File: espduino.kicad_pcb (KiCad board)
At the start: 2 copper layers, 62 x 65 mm, 29 parts, among them CON101 USB-MICRO-B, IC101 ATMEGA168-A, P101 CONN_01X12, P102 CONN_01X12, P103 FTDI, P104 CONN_01X02, P401 CONN_01X02, P402 CONN_01X02, SW101 SPST, U201 74HCT125, U202 7400, U301 LSF0204x, U302 ESP8266, U401 LD1117S12TR, U402 LD1117S33TR, X101 16Mhz

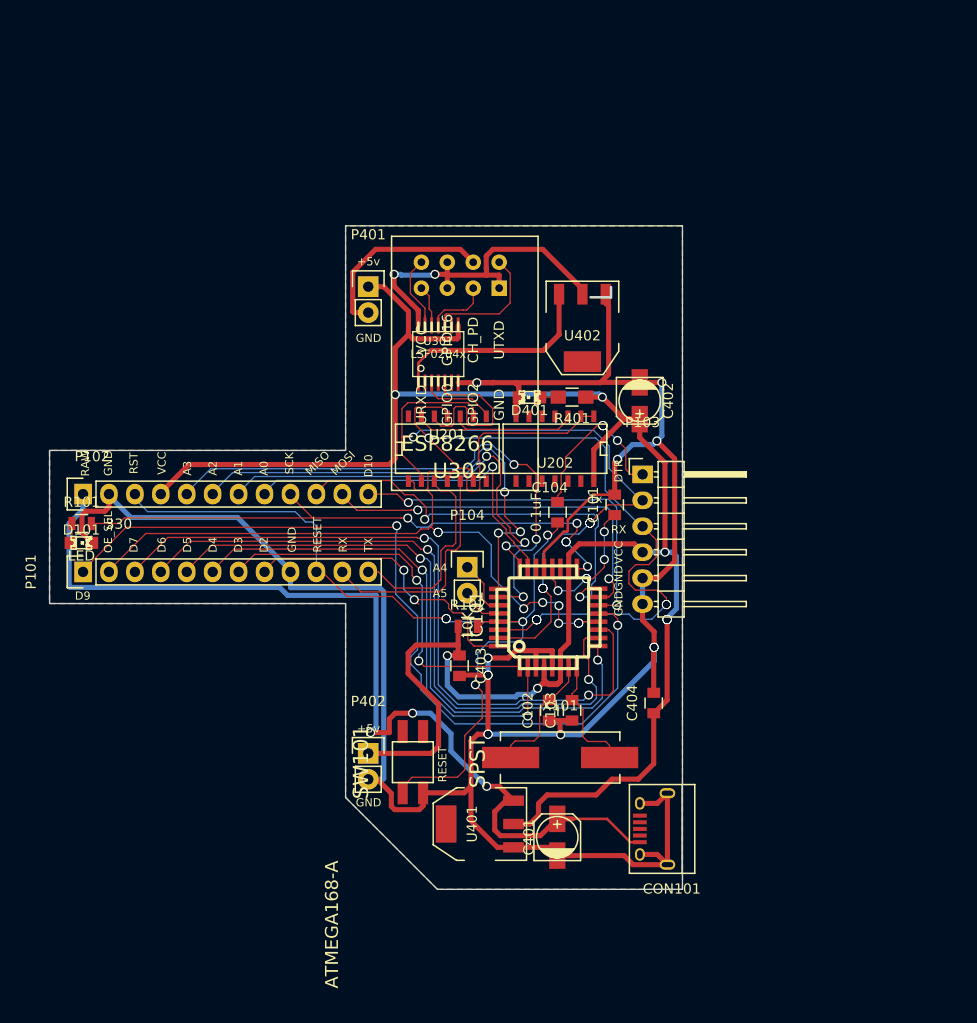
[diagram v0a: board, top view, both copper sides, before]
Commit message: More fixes
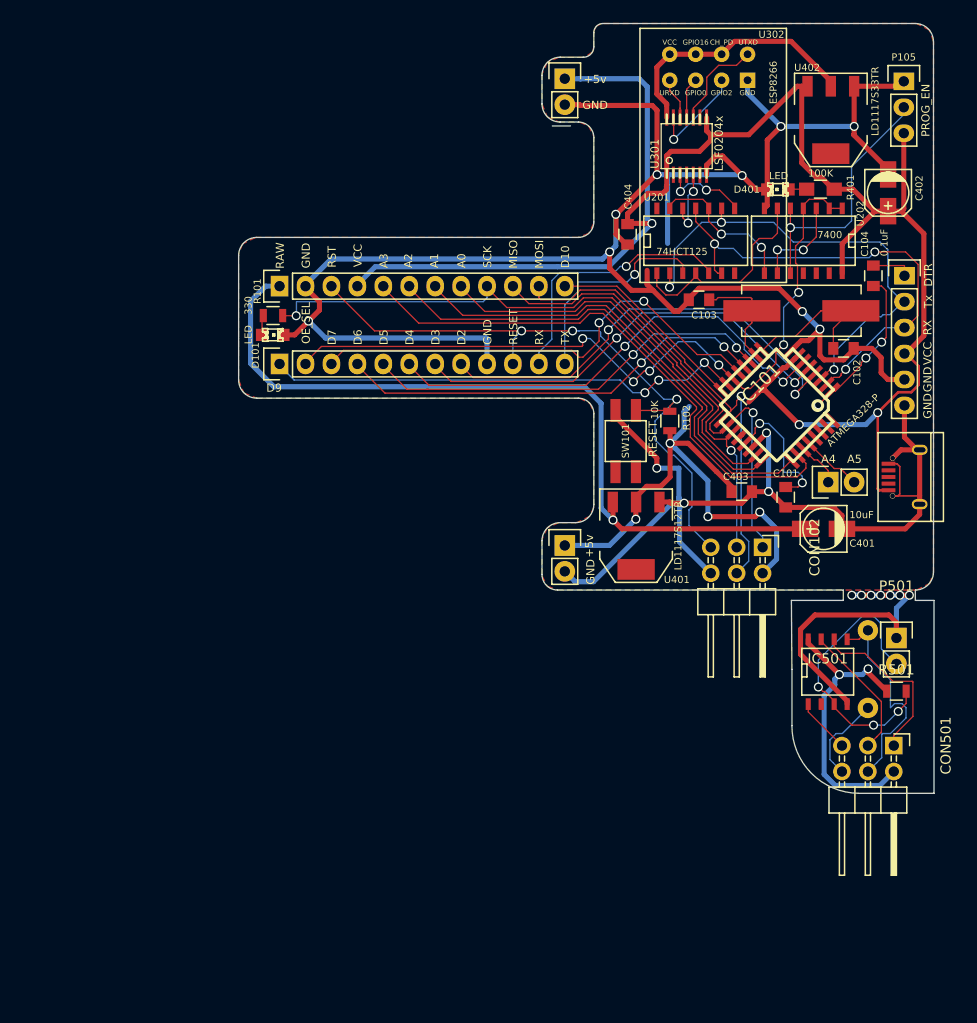
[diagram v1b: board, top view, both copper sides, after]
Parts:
- added CON102: AVR-ISP-6, Pin_Headers:Pin_Header_Angled_2x03, F.Cu at (147.9, 86.5)
- added CON501: AVR-ISP-6, Pin_Headers:Pin_Header_Angled_2x03, F.Cu at (160.7, 105.9)
- added IC501: ATTINY25-SS, SMD_Packages:SOIC-8-N, F.Cu at (154.2, 98.7)
- added P105: CONN_01X03, Pin_Headers:Pin_Header_Straight_1x03, F.Cu at (161.7, 40.8)
- added P501: CONN_01X02, Pin_Headers:Pin_Header_Straight_1x02, F.Cu at (161.0, 95.4)
- added R501: R, Resistors_SMD:R_0805, F.Cu at (161.0, 100.6)
- added SP501: SPEAKER, Buzzers_Beepers:Buzzer_12x9.5RM7.6, B.Cu at (158.2, 98.4)
- CON101: footprint Connect:USB_Micro-B -> LittlebushLogicFootPrints:USB_Micro-B
- IC101: value ATMEGA168-A -> ATMEGA328-P
- P103: footprint Pin_Headers:Pin_Header_Angled_1x06 -> Pin_Headers:Pin_Header_Straight_1x06
- U302: footprint LittlebushLogicFootPrints:ESP8266 -> LittlebushLogicFootPrints:ESP8266_2
- moved X101 49.7 mm to (151.7, 63.3), turned to 180 degrees
- moved C404 46.0 mm to (134.6, 55.8), turned to 270 degrees
- moved C102 45.7 mm to (155.8, 67.0), turned to 180 degrees
- moved CON101 44.2 mm to (161.7, 79.6), turned to 90 degrees
- moved C103 42.1 mm to (141.6, 62.2), turned to 0 degrees
- moved C401 39.9 mm to (153.8, 84.7), turned to 180 degrees
- moved C104 38.6 mm to (158.7, 59.9)
- moved SW101 37.7 mm to (134.4, 76.1), turned to 270 degrees
- moved P104 36.3 mm to (154.3, 80.1), turned to 90 degrees
- moved C403 32.5 mm to (145.8, 81.0), turned to 0 degrees
- moved P103 32.2 mm to (161.7, 59.9)
- moved U401 32.1 mm to (135.5, 85.4), turned to 180 degrees
- moved C402 31.7 mm to (160.1, 51.8)
- moved D401 31.7 mm to (149.4, 51.4)
- moved U301 31.7 mm to (140.4, 47.2)
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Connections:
- CON101 pad 1: /Voltage Regulation/RAW -> VCC
- IC101 pad 1: /D3 -> /RESET
- IC101 pad 10: /D6 -> Net-(C103-Pad2)
- IC101 pad 11: /D7 -> /D5
- IC101 pad 12: /UART Selector/OE_Sel -> /D6
- IC101 pad 13: /D9 -> /D7
- IC101 pad 14: /D10 -> /UART Selector/OE_Sel
- IC101 pad 15: /MOSI -> /D9
- IC101 pad 16: /MISO -> /D10
- IC101 pad 17: /SCK -> /MOSI
- IC101 pad 18: VCC -> /MISO
- IC101 pad 19: (no net) -> /SCK
- IC101 pad 2: /D4 -> /UART Selector/RX
- IC101 pad 20: Net-(C101-Pad1) -> VCC
- IC101 pad 21: GND -> Net-(C101-Pad1)
- IC101 pad 22: (no net) -> GND
- IC101 pad 29: /RESET -> (no net)
- IC101 pad 3: GND -> /UART Selector/TX
- IC101 pad 30: /UART Selector/RX -> (no net)
- IC101 pad 31: /UART Selector/TX -> (no net)
- IC101 pad 32: /D2 -> (no net)
- IC101 pad 4: VCC -> /D2
- IC101 pad 5: GND -> /D3
- IC101 pad 6: VCC -> /D4
- IC101 pad 7: Net-(C102-Pad2) -> VCC
- IC101 pad 8: Net-(C103-Pad2) -> GND
- IC101 pad 9: /D5 -> Net-(C102-Pad2)
- U201 pad 1: /UART Selector/OE_Sel -> Net-(U201-Pad1)
- U201 pad 4: /UART Selector/OE_Sel -> Net-(U201-Pad1)
- U202 pad 10: (no net) -> /UART Selector/~PROG_EN
- U202 pad 3: Net-(U201-Pad10) -> Net-(U202-Pad3)
- U202 pad 4: (no net) -> /UART Selector/OE_Sel
- U202 pad 5: (no net) -> /UART Selector/~PROG_EN
- U202 pad 6: (no net) -> Net-(U201-Pad1)
- U202 pad 8: (no net) -> Net-(U201-Pad10)
- U202 pad 9: (no net) -> Net-(U202-Pad3)
- U301 pad 1: +5V -> VCC
- U402 pad 3: +5V -> VCC
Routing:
- net GND: track 267.9 -> 321.5 mm, vias 12 -> 20
- net /D9: track 81.5 -> 47.3 mm, vias 2 -> 3
- net Net-(IC501-Pad3): track 0.00 -> 28.0 mm, vias 0 -> 3
- net /UART Selector/~PROG_EN: track 0.00 -> 25.9 mm, vias 0 -> 1
- net /UART Selector/RX: track 71.5 -> 46.0 mm, vias 8 -> 3
- net /D7: track 71.0 -> 47.2 mm
- net /D6: track 66.3 -> 42.7 mm
- net /D5: track 61.7 -> 40.7 mm
- net Net-(CON501-Pad4): track 0.00 -> 21.0 mm
- net /UART Selector/TX: track 68.8 -> 47.9 mm, vias 9 -> 3
- net +5V: track 20.8 -> 0.00 mm
- net +3V3: track 33.9 -> 54.5 mm
- net Net-(U201-Pad1): track 0.00 -> 20.6 mm
- net /D10: track 36.7 -> 19.7 mm, vias 2 -> 0
- net Net-(CON501-Pad1): track 0.00 -> 16.9 mm
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- removed copper zone on B.Cu, net GND
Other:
- board size 62 x 65 mm -> 68.1 x 75.4 mm
- board text added: "PROG_EN"

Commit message: Version 0.2
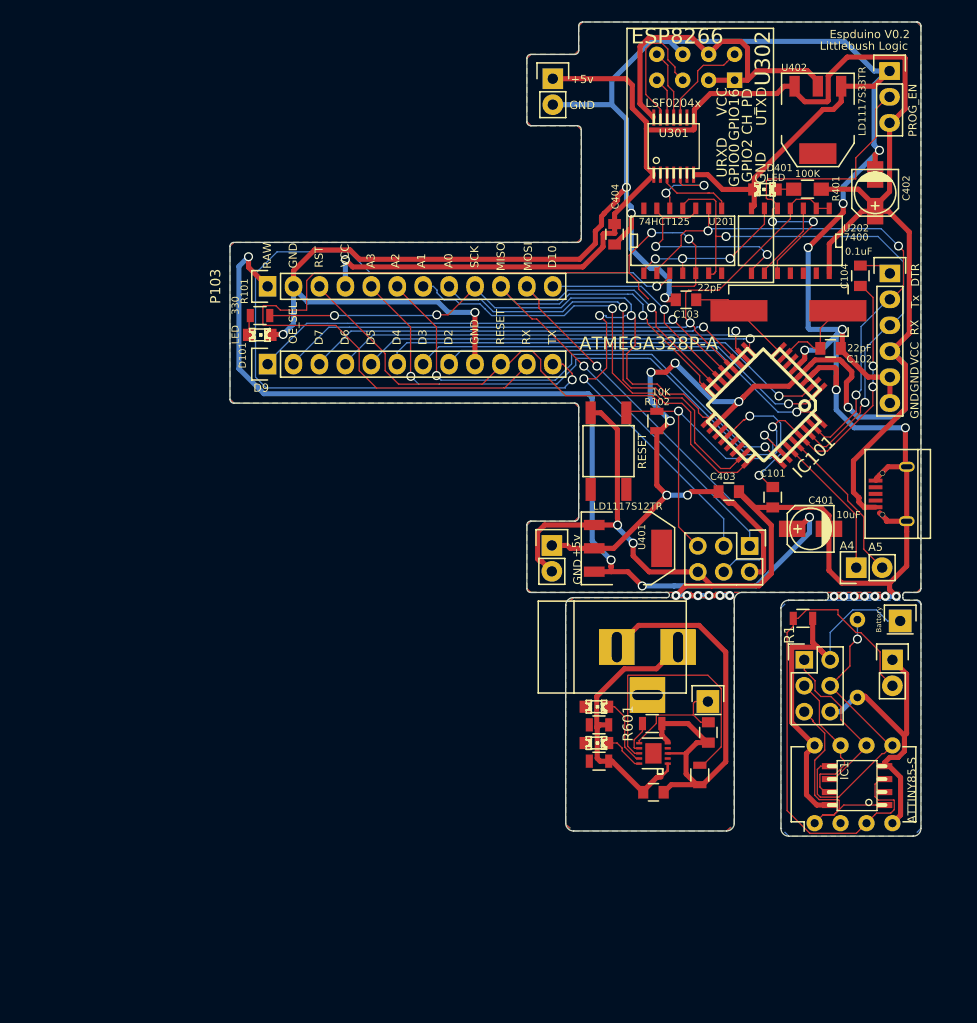
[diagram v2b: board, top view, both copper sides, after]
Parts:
- removed CON501: AVR-ISP-6, Pin_Headers:Pin_Header_Angled_2x03
- removed IC501: ATTINY25-SS, SMD_Packages:SOIC-8-N
- removed P501: CONN_01X02, Pin_Headers:Pin_Header_Straight_1x02
- removed R501: R, Resistors_SMD:R_0805
- removed SP501: SPEAKER, Buzzers_Beepers:Buzzer_12x9.5RM7.6
- added BT1: Battery, Pin_Headers:Pin_Header_Straight_1x01, F.Cu at (161.3, 93.7)
- added C601: 1uF, Capacitors_SMD:C_0805, F.Cu at (137.2, 110.5)
- added C602: 1uF, Capacitors_SMD:C_0805, F.Cu at (142.5, 104.6)
- added CON1: AVR-ISP-6, Pin_Headers:Pin_Header_Straight_2x03, F.Cu at (151.9, 97.5)
- added CON601: BARREL_JACK, Connect:BARREL_JACK, F.Cu at (133.4, 96.3)
- added D601: LED, LEDs:LED-0805, F.Cu at (131.6, 102.1)
- added D602: LED, LEDs:LED-0805, F.Cu at (131.6, 105.7)
- added IC1: ATTINY85-S, ab2_so:AB2_SO08, F.Cu at (157.1, 109.8)
- added IC2: ATTINY85-P, Housings_DIP:DIP-8_W7.62mm, F.Cu at (152.9, 113.5)
- added P1: CONN_01X02, Pin_Headers:Pin_Header_Straight_1x02, F.Cu at (160.6, 97.5)
- added P601: BATT+, Pin_Headers:Pin_Header_Straight_1x01, F.Cu at (142.5, 101.6)
- added R1: R, Resistors_SMD:R_0805, F.Cu at (151.8, 93.5)
- added R601: 10K, Resistors_SMD:R_0805, F.Cu at (137.0, 103.8)
- added R602: 1K, Resistors_SMD:R_0805, F.Cu at (131.8, 103.9)
- added R603: 1K, Resistors_SMD:R_0805, F.Cu at (131.8, 107.4)
- added R604: R, Resistors_SMD:R_0805, F.Cu at (141.7, 108.8)
- added SP1: SPEAKER, footprints:buzzer, B.Cu at (157.1, 97.4)
- added U601: LM3658, footprints:WSON10, F.Cu at (142.1, 105.2)
- CON101: footprint LittlebushLogicFootPrints:USB_Micro-B -> footprints:USB_Micro-B
- CON102: footprint Pin_Headers:Pin_Header_Angled_2x03 -> Pin_Headers:Pin_Header_Straight_2x03
- IC101: value ATMEGA328-P -> ATMEGA328P-A; footprint LittlebushLogicFootPrints:TQFP32_08 -> footprints:TQFP32_08
- P101: value CONN_01X12 -> CONN_01X03; footprint Pin_Headers:Pin_Header_Straight_1x12 -> Pin_Headers:Pin_Header_Straight_1x03
- P103: value FTDI -> CONN_01X12; footprint Pin_Headers:Pin_Header_Straight_1x06 -> Pin_Headers:Pin_Header_Straight_1x12
- P104: value CONN_01X02 -> FTDI; footprint Pin_Headers:Pin_Header_Straight_1x02 -> Pin_Headers:Pin_Header_Straight_1x06
- P105: value CONN_01X03 -> CONN_01X02; footprint Pin_Headers:Pin_Header_Straight_1x03 -> Pin_Headers:Pin_Header_Straight_1x02
- SW101: footprint LittlebushLogicFootPrints:4x4_Tactile_SMD_switch -> footprints:4x4_Tactile_SMD_switch
- U301: footprint AB2_TSSOP:AB2_TSSOP14 -> ab2_tssop:AB2_TSSOP14
- U302: footprint LittlebushLogicFootPrints:ESP8266_2 -> footprints:ESP8266_2
- moved P101 66.3 mm to (160.3, 39.8), turned to 0 degrees
- moved P103 62.4 mm to (99.4, 60.9), turned to 90 degrees
- moved P105 47.9 mm to (157.0, 88.5), turned to 90 degrees
- moved P104 21.3 mm to (160.3, 59.7), turned to 0 degrees
- moved P102 7.73 mm to (99.4, 68.5)
- moved CON101 2.09 mm to (160.5, 81.3)
- moved SW101 1.95 mm to (132.8, 77.1)
- moved U401 1.47 mm to (134.7, 86.6), turned to 270 degrees
- moved CON102 1.28 mm to (146.6, 86.4)
- moved C101 1.27 mm to (148.8, 81.6)
- moved C102 1.27 mm to (154.5, 67.0)
- moved C103 1.27 mm to (140.3, 62.2)
- moved C404 1.27 mm to (133.3, 55.8)
- moved D401 1.27 mm to (148.1, 51.4)
- moved R101 1.27 mm to (98.6, 63.8)
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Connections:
- IC101 pad 1: /RESET -> /D3
- IC101 pad 10: Net-(C103-Pad2) -> /D6
- IC101 pad 11: /D5 -> /D7
- IC101 pad 12: /D6 -> /UART Selector/OE_Sel
- IC101 pad 13: /D7 -> /D9
- IC101 pad 14: /UART Selector/OE_Sel -> /D10
- IC101 pad 15: /D9 -> /MOSI
- IC101 pad 16: /D10 -> /MISO
- IC101 pad 17: /MOSI -> /SCK
- IC101 pad 18: /MISO -> VCC
- IC101 pad 19: /SCK -> (no net)
- IC101 pad 2: /UART Selector/RX -> /D4
- IC101 pad 20: VCC -> Net-(C101-Pad1)
- IC101 pad 21: Net-(C101-Pad1) -> (no net)
- IC101 pad 22: GND -> (no net)
- IC101 pad 29: (no net) -> /RESET
- IC101 pad 3: /UART Selector/TX -> GND
- IC101 pad 30: (no net) -> /UART Selector/RX
- IC101 pad 31: (no net) -> /UART Selector/TX
- IC101 pad 32: (no net) -> /D2
- IC101 pad 4: /D2 -> VCC
- IC101 pad 5: /D3 -> GND
- IC101 pad 6: /D4 -> (no net)
- IC101 pad 7: VCC -> Net-(C102-Pad2)
- IC101 pad 8: GND -> Net-(C103-Pad2)
- IC101 pad 9: Net-(C102-Pad2) -> /D5
- P101 pad 1: /D9 -> GND
- P101 pad 2: /UART Selector/OE_Sel -> /UART Selector/~PROG_EN
- P101 pad 3: /D7 -> VCC
- P102 pad 1: /Voltage Regulation/RAW -> /D9
- P102 pad 10: /MISO -> /RESET
- P102 pad 11: /MOSI -> /UART Selector/RX_1
- P102 pad 12: /D10 -> /UART Selector/TX_1
- P102 pad 2: GND -> /UART Selector/OE_Sel
- P102 pad 3: /RESET -> /D7
- P102 pad 4: VCC -> /D6
- P102 pad 5: /A3 -> /D5
- P102 pad 6: /A2 -> /D4
- P102 pad 7: /A1 -> /D3
- P102 pad 8: /A0 -> /D2
- P102 pad 9: /SCK -> GND
- P103 pad 1: /DTR -> /Voltage Regulation/RAW
- P103 pad 2: /UART Selector/TX -> GND
- P103 pad 3: /UART Selector/RX -> /RESET
- P103 pad 5: GND -> /A3
- P103 pad 6: GND -> /A2
- P104 pad 1: /A4 -> /DTR
- P104 pad 2: /A5 -> /UART Selector/TX
- P105 pad 1: GND -> /A4
- P105 pad 2: /UART Selector/~PROG_EN -> /A5
- U302 pad 2: GND -> +3V3
- U302 pad 4: Net-(U301-Pad13) -> +3V3
- U302 pad 5: +3V3 -> GND
- U302 pad 6: Net-(U301-Pad11) -> Net-(U301-Pad13)
- U302 pad 7: +3V3 -> Net-(U301-Pad11)
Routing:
- net GND: track 321.5 -> 431.1 mm, vias 20 -> 27
- net /UART Selector/TX_1: track 21.7 -> 88.6 mm, vias 1 -> 2
- net /UART Selector/RX_1: track 26.2 -> 91.1 mm, vias 1 -> 2
- net /Freezy/ADC: track 0.00 -> 51.4 mm
- net Net-(BT1-Pad1): track 0.00 -> 38.3 mm
- net /Freezy/MOSI: track 0.00 -> 29.4 mm, vias 0 -> 1
- net Net-(IC501-Pad3): track 28.0 -> 0.00 mm, vias 3 -> 0
- net +6V: track 0.00 -> 27.2 mm
- net Net-(R604-Pad2): track 0.00 -> 26.6 mm
- net /Freezy/~RST: track 0.00 -> 22.3 mm
- net /RESET: track 80.9 -> 102.4 mm, vias 6 -> 4
- net VCC: track 224.3 -> 245.4 mm, vias 7 -> 8
- net Net-(CON501-Pad4): track 21.0 -> 0.00 mm
- net /SCK: track 69.0 -> 89.6 mm, vias 2 -> 5
- net +3V3: track 54.5 -> 35.0 mm, vias 2 -> 0
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- added copper zone on B.Cu, net GND
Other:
- board size 68.1 x 75.4 mm -> 67.7 x 79.8 mm
- net class Charger added: clearance 0.127, trace_width 0.127, via_dia 0.889, via_drill 0.635
- net class Default: clearance 0.254 -> 0.127
- net class Power: clearance 0.254 -> 0.127
- rule trace_clearance: 0.254 -> 0.127
- board text added: "Espduino V0.2"
- board text added: "Littlebush Logic"
